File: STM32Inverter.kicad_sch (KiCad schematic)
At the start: 99 parts, among them J1 STLINK, J2 CURRENT SENSE, J5 UART, J6 INTERFACE, J7 POWER, J8 501571-2007, J9 RESOLVER, Q4 ST3422A, U1 STM32F303VCTx, U10 ULN2002, U11 LM393, U12 LM393, U4 74HCT00, U7 MCP2551-I-SN, Y3 CSTNE8M00GH5C000R0

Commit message: Resolver layout
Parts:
- J2: footprint DF51K4P2DS805 -> DF51-4:DF51K4P2DS805
- J7: footprint DF51K8DP2DS805 -> DF51-8:DF51K8DP2DS805
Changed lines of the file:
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@@
       (effects (font (size 1.27 1.27)))
     )
-    (property "Footprint" "DF51K4P2DS805" (at 20.32 215.57 0)
+    (property "Footprint" "DF51-4:DF51K4P2DS805" (at 20.32 215.57 0)
       (effects (font (size 1.27 1.27)) (justify left top) hide)
     )
@@
       (effects (font (size 1.27 1.27)))
     )
-    (property "Footprint" "DF51K8DP2DS805" (at 63.5 395.91 0)
+    (property "Footprint" "DF51-8:DF51K8DP2DS805" (at 63.5 395.91 0)
       (effects (font (size 1.27 1.27)) (justify left top) hide)
     )

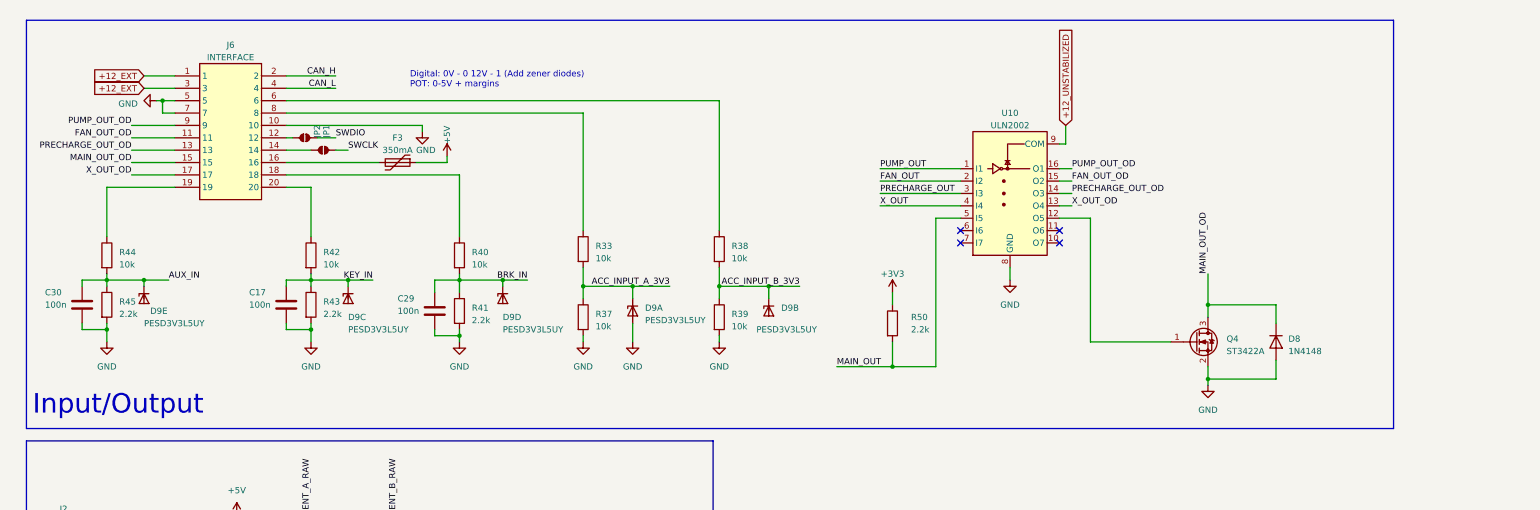
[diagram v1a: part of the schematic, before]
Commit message: Layout mostly done
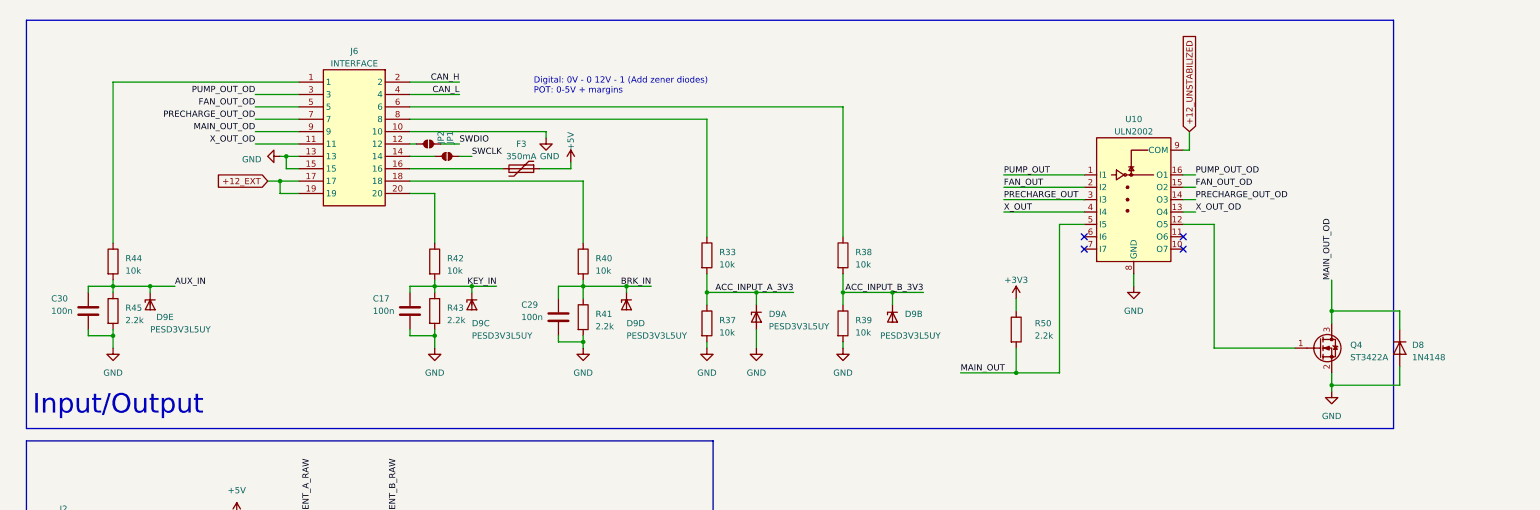
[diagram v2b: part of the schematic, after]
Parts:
- U11, U12: footprint Package_SO:SOP-8_3.9x4.9mm_P1.27mm -> Package_SO:SO-8_3.9x4.9mm_P1.27mm
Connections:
- net +12_EXT: now also J6.17, J6.19; no longer J6.1, J6.3
- net FAN_OUT_OD: now also J6.5; no longer J6.11
- net GND: now also J6.13, J6.15; no longer J6.5, J6.7
- net MAIN_OUT_OD: now also J6.9; no longer J6.15
- net PRECHARGE_OUT_OD: now also J6.7; no longer J6.13
- net PUMP_OUT_OD: now also J6.3; no longer J6.9
- net X_OUT_OD: now also J6.11; no longer J6.17
- net at R44.1: now also J6.1; no longer J6.19
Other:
- moved on the sheet: C17, C29, D8, D9A, D9B, D9C, D9D, F3, J6, JP1, JP2, Q4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
